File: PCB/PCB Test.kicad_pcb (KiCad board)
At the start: 2 copper layers, 51.7 x 63.4 mm, 49 parts, among them J1 Conn_02x02_Odd_Even, J2 Conn_02x05_Odd_Even, J3 Conn_02x02_Counter_Clockwise, J4 Conn_02x02_Counter_Clockwise, J5 Conn_02x02_Counter_Clockwise, J6 Conn_02x03_Odd_Even, Q2 NMOS, Q3 NMOS, U1 ATmega4808-A, U5 MCP1700x-330xxTO

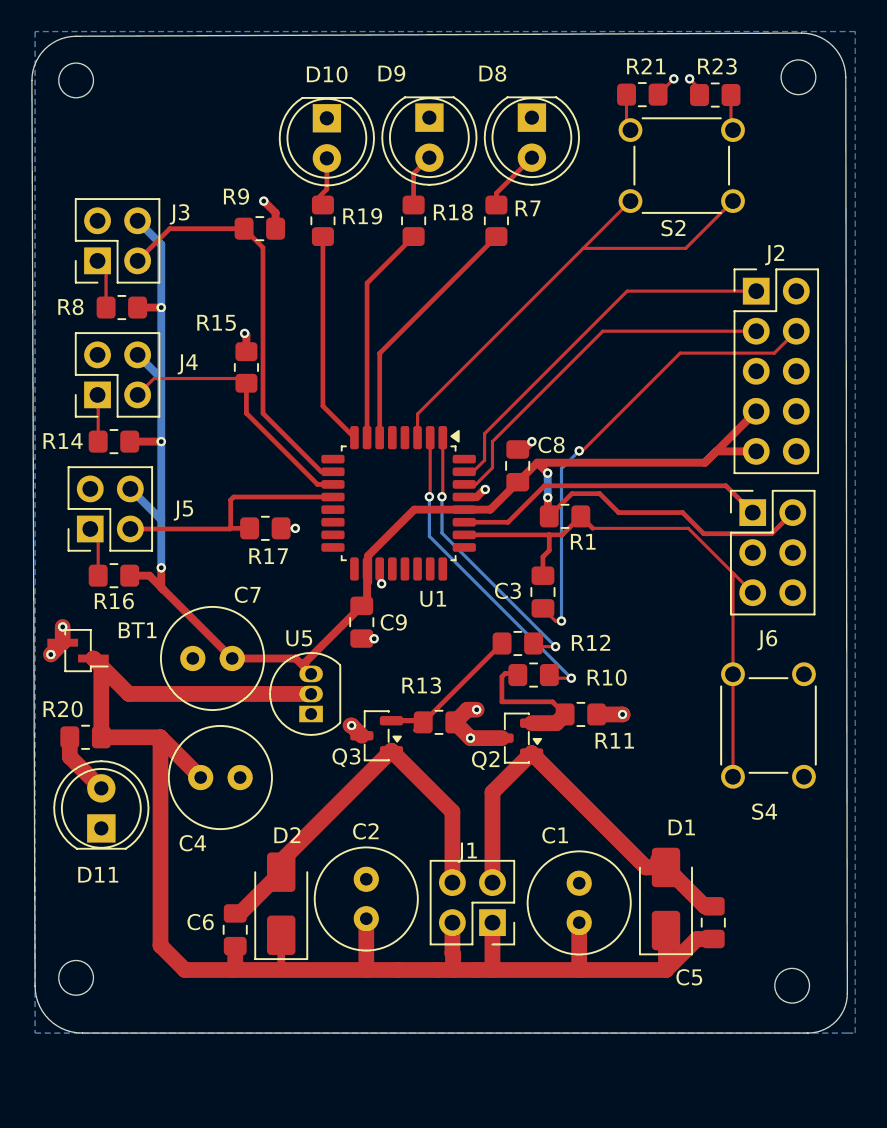
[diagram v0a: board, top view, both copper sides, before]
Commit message: Final touches, v1 is ready
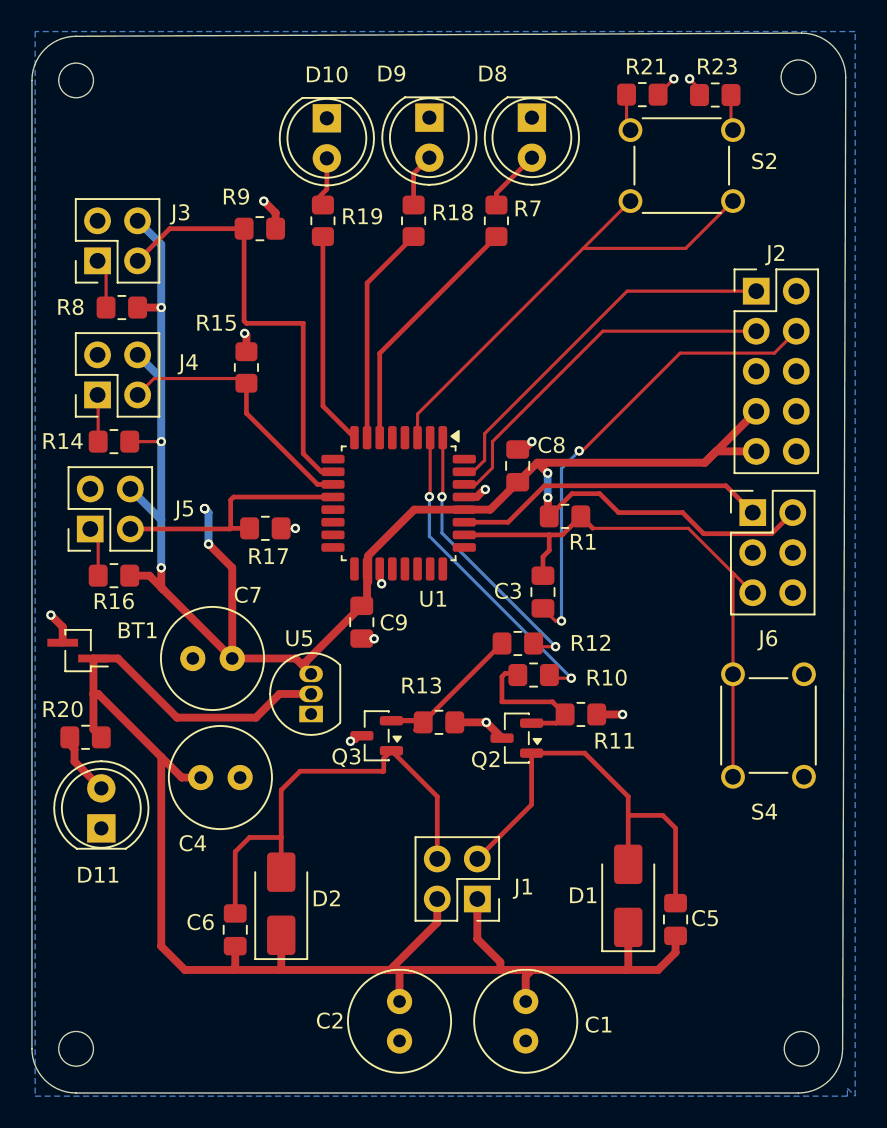
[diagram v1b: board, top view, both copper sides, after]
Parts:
- moved C1 10.6 mm to (164.1, 152.5), turned to 90 degrees
- moved C2 10.5 mm to (156.1, 152.5), turned to 90 degrees
- moved H4 4.50 mm to (135.6, 153.0)
- moved H3 4.04 mm to (181.6, 153.0)
- moved C5 2.40 mm to (173.6, 144.8)
- moved D1 2.40 mm to (170.6, 143.3)
- moved J1 1.78 mm to (161.0, 143.5)
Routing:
- net +3.3V: track 109.9 -> 120.2 mm, vias 5 -> 8
- net Net-(D2-A): track 24.6 -> 29.0 mm
- net +4.8V: track 95.6 -> 98.6 mm
- net Net-(D1-A): track 25.5 -> 27.8 mm
- net ADC Sensor 3: track 25.8 -> 27.9 mm
- net GND: track 21.6 -> 19.7 mm, vias 15 -> 13
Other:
- board size 51.7 x 63.4 mm -> 51.6 x 67.2 mm
- board text added: "Peter Ladur Line Following Robot"
- board text removed: "LAB_A/01 B: Peter, Arinze, Antoine, Ollie"
- board text removed: "V1"
